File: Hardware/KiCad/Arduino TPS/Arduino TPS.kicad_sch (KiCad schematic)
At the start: 21 parts, among them SW1 SW_Push, SW2 SW_Push, SW3 SW_Push, SW4 SW_Push, SW5 SW_Push, SW6 SW_Push

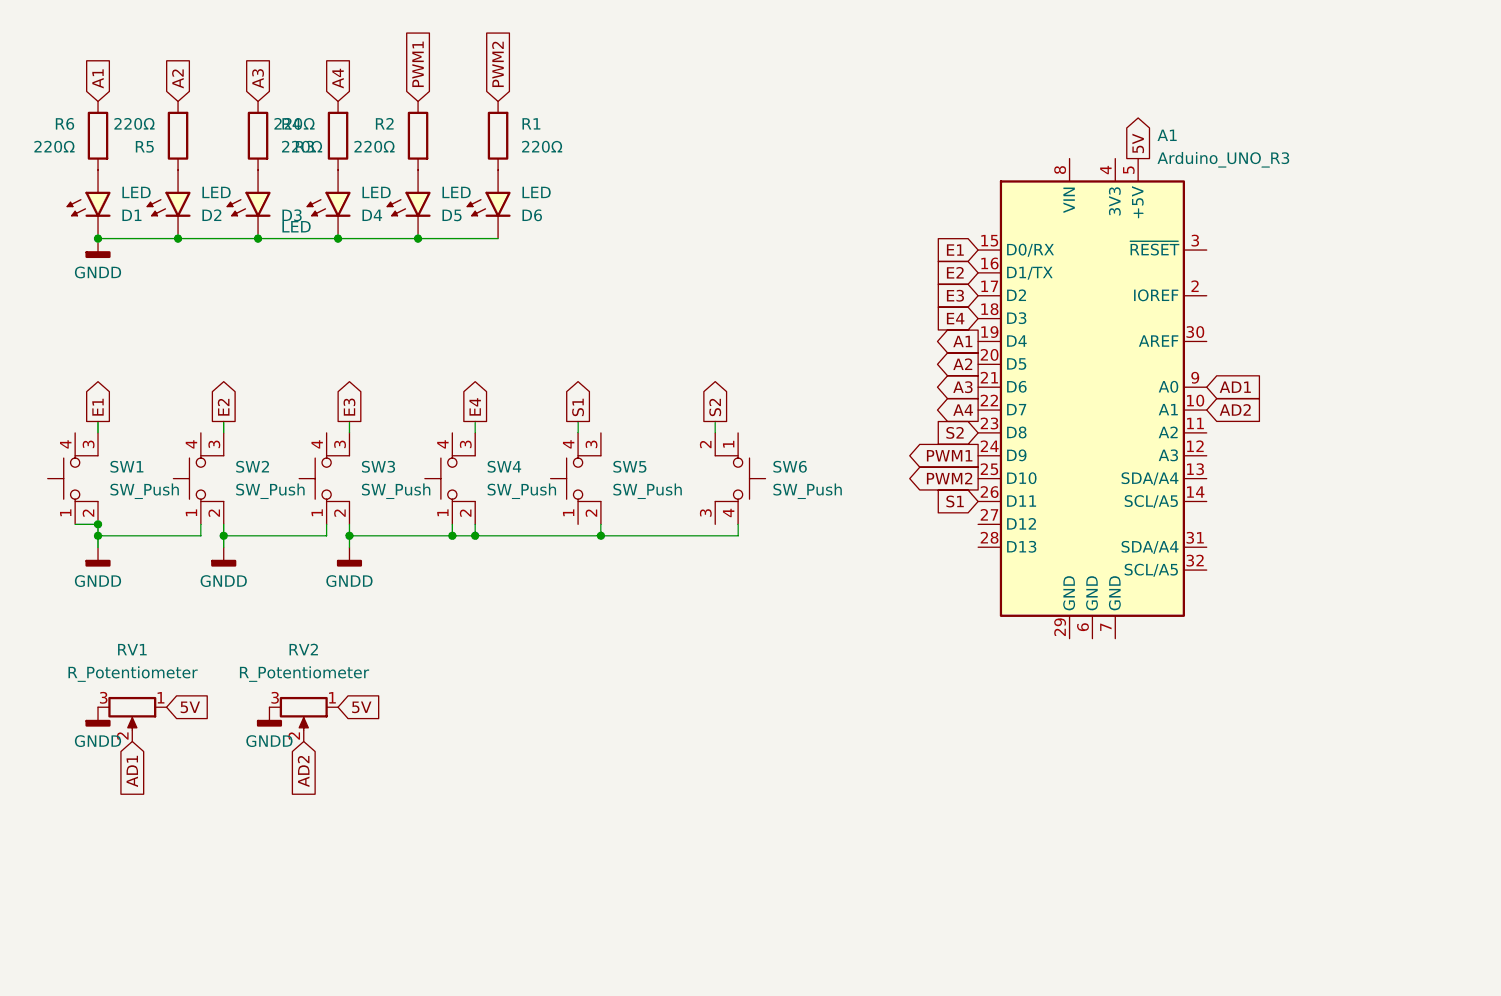
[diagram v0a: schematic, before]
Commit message: Update
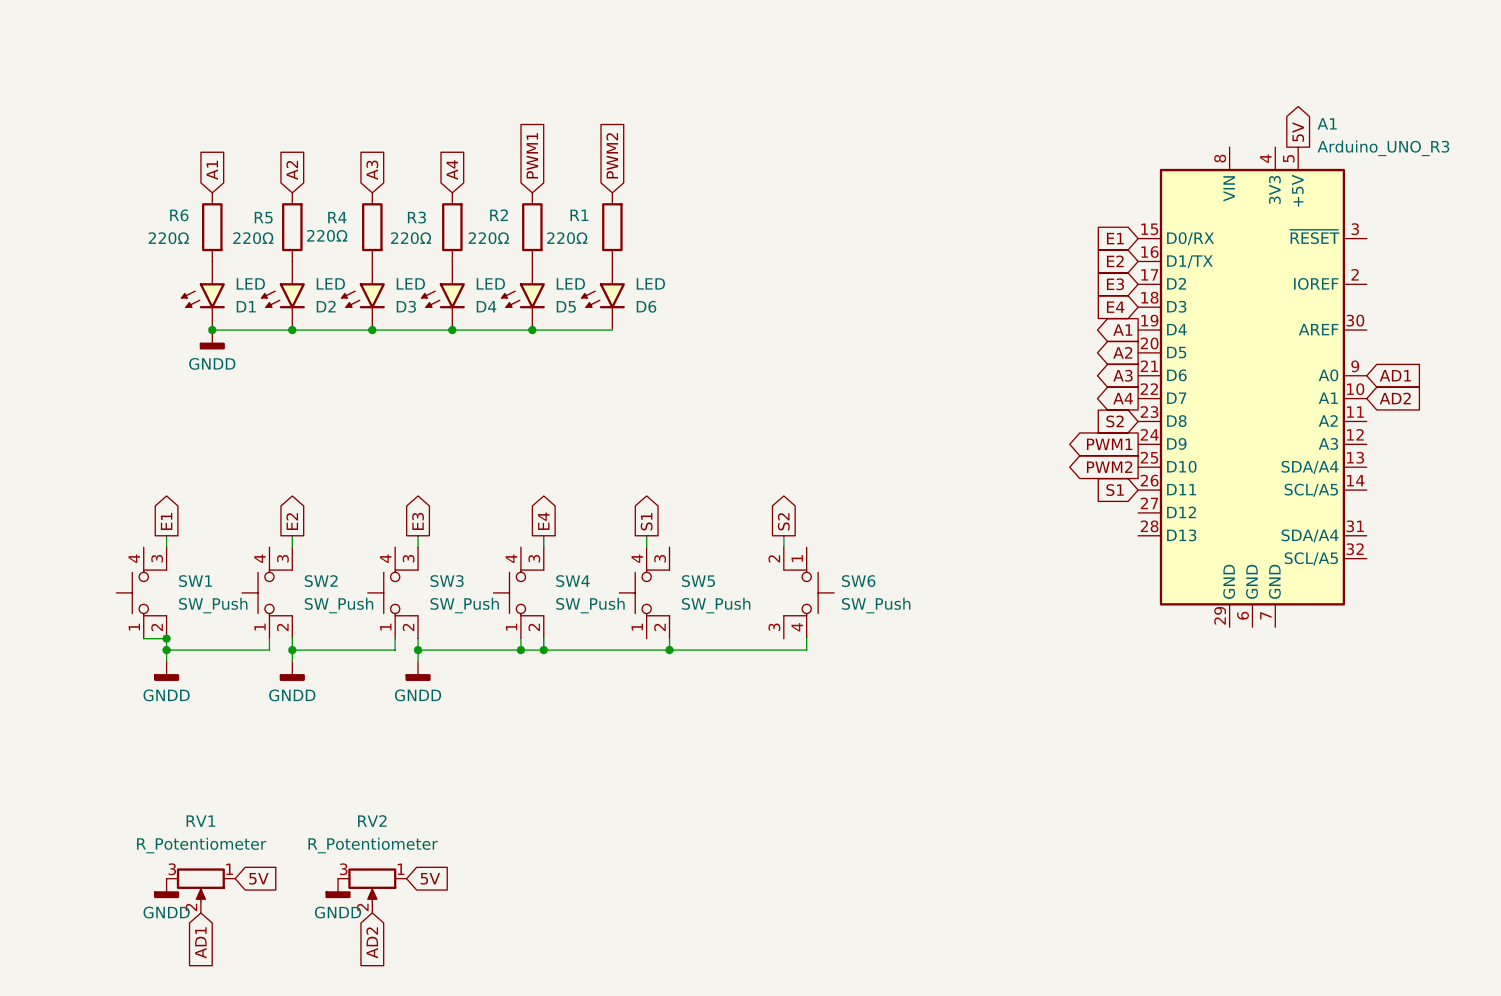
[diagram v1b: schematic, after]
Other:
- moved on the sheet: A1, D1, D2, D3, D4, D5, D6, R1, R2, R3, R4, R5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
